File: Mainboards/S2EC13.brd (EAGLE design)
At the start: 43 x 72 mm, 52 parts, among them IC1 LD1117S33, IC2 CC1101RTK, IC3 STM32F051C8, Q1 IRLML9301, Q2 8M, X1 VCC, X2 CLK, X3 GND, X4 DIO, X5 RST, X6 NC

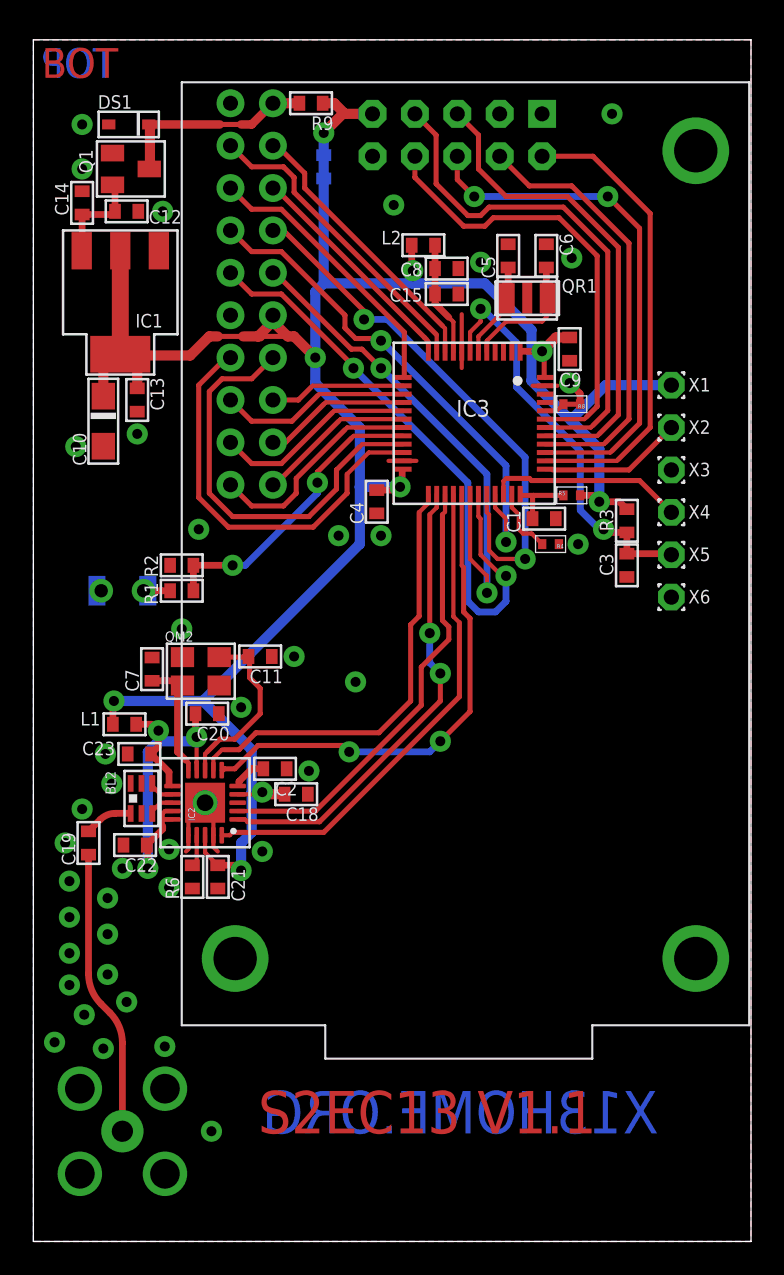
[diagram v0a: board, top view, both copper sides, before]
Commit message: S2ER13 Proto
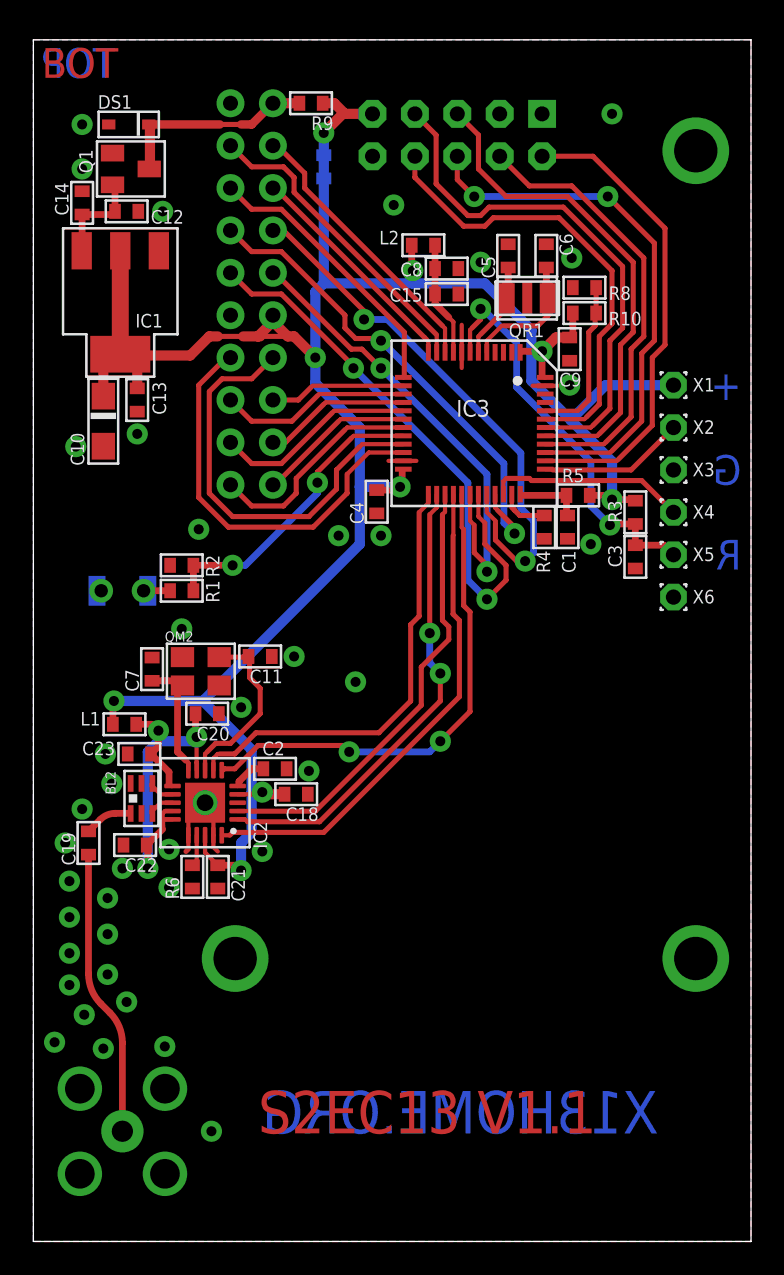
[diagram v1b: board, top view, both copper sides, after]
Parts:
- added R10: NC, RCL:0603
- R4, R5: device RCL:0402 -> RCL:0603
- R8: value 0R -> 10k; device RCL:0402 -> RCL:0603
- moved R8 7.03 mm to (33.0, 57.1), turned to 0 degrees
- moved C1 1.49 mm to (32.0, 42.8), turned to 270 degrees
- moved R4 1.09 mm to (30.6, 42.8), turned to 90 degrees
- moved C3 0.72 mm to (36.1, 41.0)
- moved R3 0.72 mm to (36.1, 43.7)
- moved R5 0.38 mm to (32.6, 44.7)
- moved X1 0.13 mm to (38.4, 51.3)
- moved X2 0.13 mm to (38.4, 48.8)
- moved X3 0.13 mm to (38.4, 46.2)
- moved X4 0.13 mm to (38.4, 43.7)
- moved X5 0.13 mm to (38.4, 41.1)
- moved X6 0.13 mm to (38.4, 38.6)
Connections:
- net +3V3: now also R10.1
- net BOOT0: now also R10.2
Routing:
- net BOOT0: track 1.25 -> 9.79 mm
- net PA9: track 31.3 -> 28.7 mm
- net PA10: track 36.8 -> 34.4 mm
- net GND: track 13.0 -> 10.8 mm
- net +3V3: track 145.7 -> 147.3 mm
- net N$2: track 4.05 -> 2.93 mm
- net N$5: track 1.02 -> 0.00 mm
- net L_RST/RX1: track 27.1 -> 27.9 mm
- net L_MOSI: track 29.1 -> 29.8 mm
- net L_MISO: track 26.1 -> 26.8 mm
- net L_SCK: track 31.6 -> 32.3 mm
- net L_IRQ: track 27.8 -> 28.6 mm
- net L_SEL/TX1: track 30.8 -> 31.5 mm
- net PA12: track 30.5 -> 29.9 mm
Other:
- board text added: "+"
- board text added: "G"
- board text added: "R"
